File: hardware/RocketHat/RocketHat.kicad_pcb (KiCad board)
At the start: 4 copper layers, 28 x 25 mm, 32 parts, among them J1 Conn_02x16_Top_Bottom, J2 Conn_02x16_Top_Bottom, Q2 MMBT2222A, U1 BMP390, U2 BMI088, U3 ADXL375BCCZ, U5 74HC688, U6 74HC245, U7 74HC245, U8 MAX-M10S

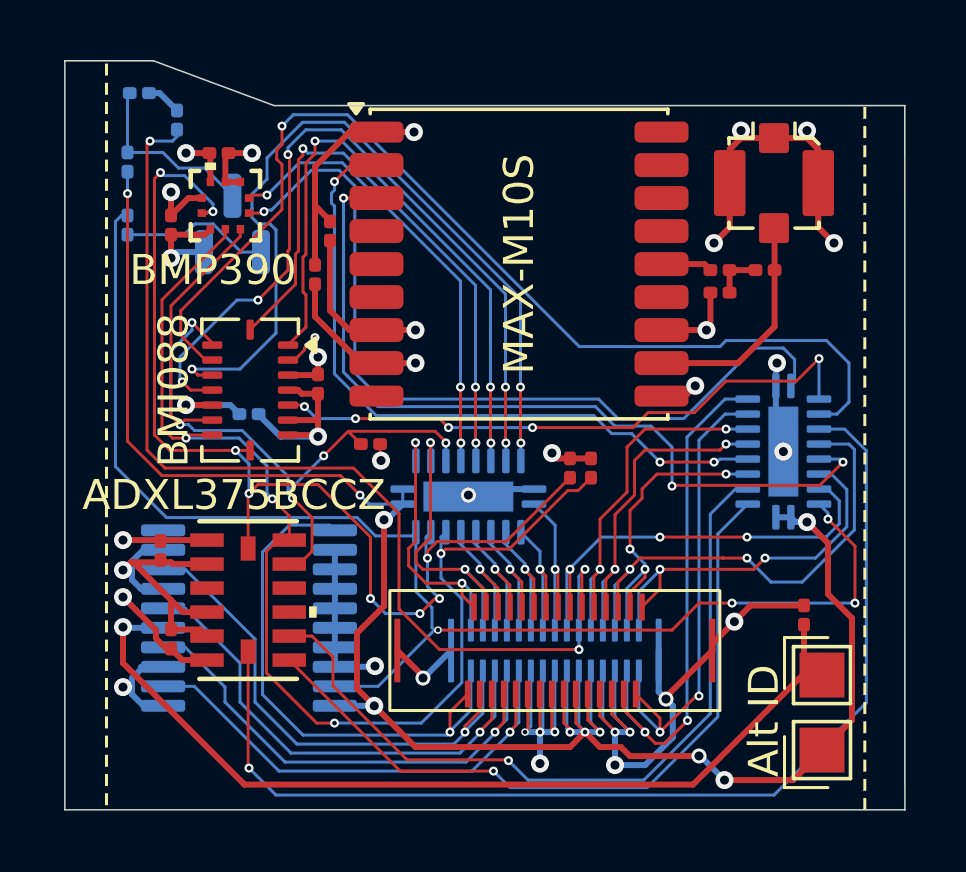
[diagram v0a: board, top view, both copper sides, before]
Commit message: sanity checked, ready for production
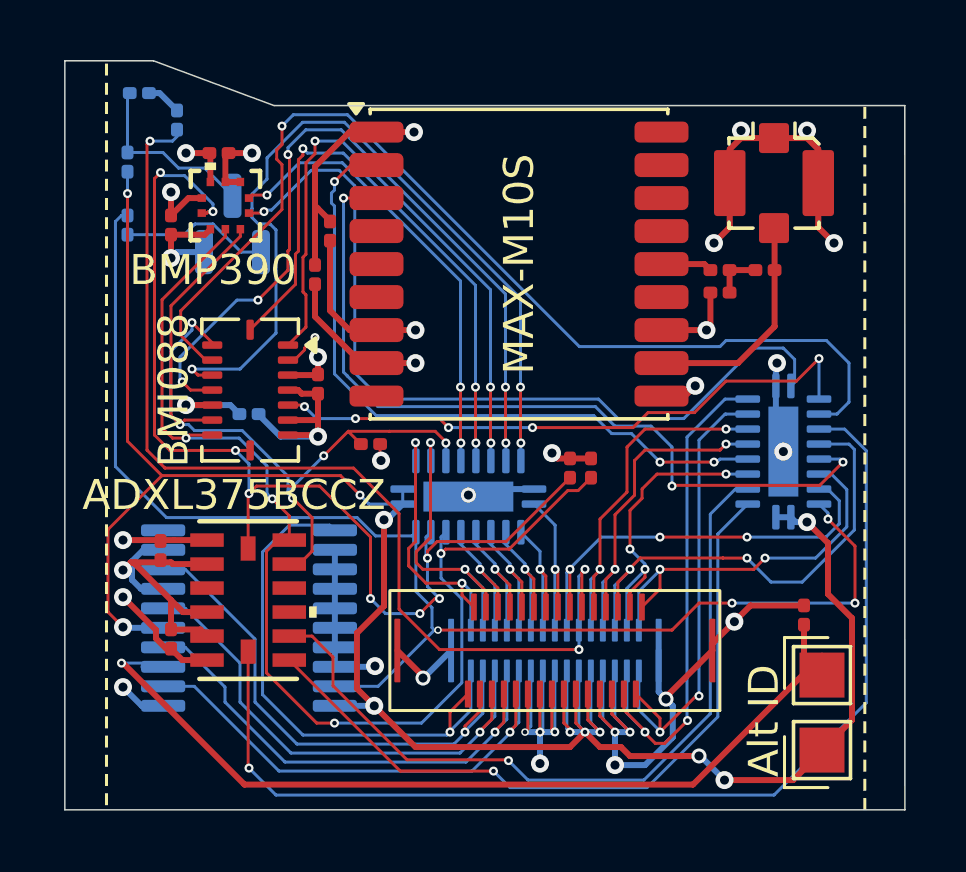
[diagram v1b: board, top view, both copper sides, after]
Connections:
- R8 pad 1: Net-(U5-R1) -> Net-(U5-R0)
- TP1 pad 1: Net-(U5-R1) -> Net-(U5-R0)
- U5 pad 3: CONN_26/GND -> Net-(U5-R0)
- U5 pad 5: Net-(U5-R1) -> CONN_23/5V
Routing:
- net Net-(U5-R1): track 31.2 -> 0.00 mm, vias 1 -> 0
- net Net-(U5-R0): track 0.00 -> 30.8 mm, vias 0 -> 1
- net CONN_23/5V: track 66.8 -> 74.2 mm, vias 10 -> 11
- net CONN_26/GND: track 87.4 -> 85.7 mm
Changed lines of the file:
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@@
 	(net 59 "CONN_2{slash}D2")
 	(net 60 "CONN_4{slash}D4")
-	(net 61 "Net-(U5-R1)")
+	(net 61 "Net-(U5-R0)")
 	(footprint "Capacitor_SMD:C_0201_0603Metric"
 		(layer "F.Cu")
@@
 			(size 1.5 1.5)
 			(layers "F.Cu" "F.Mask")
-			(net 61 "Net-(U5-R1)")
+			(net 61 "Net-(U5-R0)")
 			(pinfunction "1")
 			(pintype "passive")
@@
 			(layers "F.Cu" "F.Mask")
 			(roundrect_rratio 0.25)
-			(net 61 "Net-(U5-R1)")
+			(net 61 "Net-(U5-R0)")
 			(pintype "passive")
 		)
@@
 			(layers "B.Cu" "B.Mask" "B.Paste")
 			(roundrect_rratio 0.25)
-			(net 1 "CONN_26{slash}GND")
+			(net 61 "Net-(U5-R0)")
 			(pinfunction "R0")
 			(pintype "input")
@@
 			(layers "B.Cu" "B.Mask" "B.Paste")
 			(roundrect_rratio 0.25)
-			(net 61 "Net-(U5-R1)")
+			(net 5 "CONN_23{slash}5V")
 			(pinfunction "R1")
 			(pintype "input")
@@
 	)
 	(segment
-		(start 130.599 116.04387)
-		(end 130.599 115.8)
-		(width 0.2)
-		(layer "B.Cu")
-		(net 1)
-	)
-	(segment
 		(start 146.7 117.3)
 		(end 146.7 118.4)
@@
 	)
 	(segment
-		(start 130.599 115.8)
-		(end 130.3 115.8)
-		(width 0.2)
-		(layer "B.Cu")
-		(net 1)
-	)
-	(segment
 		(start 152.3125 107.95)
 		(end 152.0625 107.7)
@@
 	)
 	(segment
-		(start 130.599 115.50613)
-		(end 130.98013 115.125)
+		(start 147.702455 118.4)
+		(end 148.626 117.476455)
 		(width 0.2)
 		(layer "B.Cu")
@@
 	)
 	(segment
-		(start 147.702455 118.4)
-		(end 148.626 117.476455)
+		(start 131.6375 116.425)
+		(end 130.98013 116.425)
 		(width 0.2)
 		(layer "B.Cu")
@@
 	(segment
 		(start 131.6375 116.425)
-		(end 130.98013 116.425)
+		(end 130.925 116.425)
 		(width 0.2)
 		(layer "B.Cu")
@@
 	)
 	(segment
-		(start 130.98013 115.125)
-		(end 131.6375 115.125)
+		(start 130.925 116.425)
+		(end 130.3 115.8)
 		(width 0.2)
 		(layer "B.Cu")
@@
 	)
 	(segment
-		(start 131.6375 115.125)
-		(end 130.900001 115.125)
-		(width 0.2)
-		(layer "B.Cu")
-		(net 1)
-	)
-	(segment
 		(start 130.599 112.223999)
 		(end 130.599 111.9)
@@
 	)
 	(segment
-		(start 130.599 115.8)
-		(end 130.599 115.50613)
-		(width 0.2)
-		(layer "B.Cu")
-		(net 1)
-	)
-	(segment
 		(start 138.675 115.125)
 		(end 138.7 115.1)
@@
 	)
 	(segment
-		(start 130.98013 116.425)
-		(end 130.599 116.04387)
-		(width 0.2)
-		(layer "B.Cu")
-		(net 1)
-	)
-	(segment
 		(start 146.7 118.4)
 		(end 147.702455 118.4)
@@
 	)
 	(segment
+		(start 129.799 113.299)
+		(end 130.3 113.8)
+		(width 0.1)
+		(layer "F.Cu")
+		(net 5)
+	)
+	(segment
 		(start 130.45 107.604968)
 		(end 131.596032 108.751)
@@
 	)
 	(segment
+		(start 131.596032 108.751)
+		(end 129.799 110.548032)
+		(width 0.1)
+		(layer "F.Cu")
+		(net 5)
+	)
+	(segment
 		(start 147.2 118.1)
 		(end 146.899 117.799)
@@
 	)
 	(segment
+		(start 129.799 110.548032)
+		(end 129.799 113.299)
+		(width 0.1)
+		(layer "F.Cu")
+		(net 5)
+	)
+	(segment
 		(start 145.7953 116.8953)
 		(end 146.2 117.3)
@@
 	)
 	(via
+		(at 130.3 113.8)
+		(size 0.6)
+		(drill 0.3)
+		(layers "F.Cu" "B.Cu")
+		(net 5)
+	)
+	(via
 		(at 145.2 117.3)
 		(size 0.3)
@@
 	)
 	(segment
+		(start 130.325 113.825)
+		(end 130.3 113.8)
+		(width 0.2)
+		(layer "B.Cu")
+		(net 5)
+	)
+	(segment
 		(start 152.5625 110.1375)
 		(end 152.0625 110.1375)
@@
 	)
 	(segment
+		(start 131.6375 113.825)
+		(end 130.325 113.825)
+		(width 0.2)
+		(layer "B.Cu")
+		(net 5)
+	)
+	(segment
 		(start 152.5625 110.1375)
 		(end 152.725 110.3)
@@
 	)
 	(segment
+		(start 138.55 110.8)
+		(end 138.55 112.85)
+		(width 0.1)
+		(layer "F.Cu")
+		(net 25)
+	)
+	(segment
 		(start 140.45 111.268255)
 		(end 140.768255 110.95)
@@
 	)
 	(segment
+		(start 134.5 109.35)
+		(end 134.75 109.1)
+		(width 0.1)
+		(layer "F.Cu")
+		(net 25)
+	)
+	(segment
 		(start 131.55 98.65)
 		(end 131.35 98.85)
@@
 	)
 	(segment
-		(start 134.8 109.05)
-		(end 136.8 109.05)
-		(width 0.1)
-		(layer "F.Cu")
-		(net 25)
-	)
-	(segment
 		(start 140.768255 110.95)
 		(end 143.07 110.95)
@@
 	)
 	(segment
-		(start 134.5 109.35)
-		(end 134.8 109.05)
+		(start 134.75 109.1)
+		(end 136.85 109.1)
 		(width 0.1)
 		(layer "F.Cu")
@@
 	)
 	(segment
-		(start 136.8 109.05)
+		(start 136.85 109.1)
 		(end 138.55 110.8)
 		(width 0.1)
@@
 	)
 	(segment
-		(start 138.55 110.8)
-		(end 138.55 112.85)
-		(width 0.1)
-		(layer "F.Cu")
-		(net 25)
-	)
-	(segment
 		(start 131.35 107.4)
 		(end 131.8625 107.9125)
@@
 	)
 	(segment
-		(start 141.5943 115.650315)
-		(end 141.5943 112.863488)
+		(start 140.25 117)
+		(end 141.5943 115.6557)
 		(width 0.1)
 		(layer "B.Cu")
@@
 	)
 	(segment
-		(start 135.1 108.430755)
-		(end 134.169245 107.5)
+		(start 141.5943 112.863488)
+		(end 140.9 112.169188)
 		(width 0.1)
 		(layer "B.Cu")
@@
 	)
 	(segment
-		(start 135.1 109.35)
-		(end 135.1 108.430755)
+		(start 135.1 108.430755)
+		(end 134.169245 107.5)
 		(width 0.1)
 		(layer "B.Cu")
@@
 	)
 	(segment
-		(start 140.244615 117)
-		(end 141.5943 115.650315)
+		(start 135.1 109.35)
+		(end 135.1 108.430755)
 		(width 0.1)
 		(layer "B.Cu")
@@
 	)
 	(segment
-		(start 140.9 111.35)
-		(end 140.9 110.8)
+		(start 141.5943 115.6557)
+		(end 141.5943 112.863488)
 		(width 0.1)
 		(layer "B.Cu")
@@
 	)
 	(segment
-		(start 137.35 117)
-		(end 140.244615 117)
+		(start 140.9 112.169188)
+		(end 140.9 111.35)
 		(width 0.1)
 		(layer "B.Cu")
@@
 	)
 	(segment
-		(start 140.9 112.169188)
-		(end 140.9 111.35)
+		(start 140.9 111.35)
+		(end 140.9 110.8)
 		(width 0.1)
 		(layer "B.Cu")
@@
 	)
 	(segment
-		(start 141.5943 112.863488)
-		(end 140.9 112.169188)
+		(start 137.35 117)
+		(end 140.25 117)
 		(width 0.1)
 		(layer "B.Cu")
@@
 	)
 	(segment
-		(start 130.3 115)
-		(end 130.3 113.8)
+		(start 153 113.72)
+		(end 153 114.8)
 		(width 0.2)
 		(layer "F.Cu")
@@
 	)
 	(segment
-		(start 153 113.72)
-		(end 153 114.8)
-		(width 0.2)
+		(start 130.3 115)
+		(end 130.25 115)
+		(width 0.1)
 		(layer "F.Cu")
 		(net 61)
@@
 	)
 	(via
-		(at 130.3 113.8)
-		(size 0.6)
-		(drill 0.3)
+		(at 130.25 115)
+		(size 0.3)
+		(drill 0.15)
 		(layers "F.Cu" "B.Cu")
 		(net 61)
 	)
 	(segment
-		(start 130.325 113.825)
-		(end 130.3 113.8)
-		(width 0.2)
+		(start 130.25 115)
+		(end 131.5125 115)
+		(width 0.1)
 		(layer "B.Cu")
 		(net 61)
 	)
 	(segment
-		(start 131.6375 113.825)
-		(end 130.325 113.825)
+		(start 131.5125 115)
+		(end 131.6375 115.125)
+		(width 0.1)
+		(layer "B.Cu")
+		(net 61)
+	)
+	(segment
+		(start 130.98013 115.125)
+		(end 131.6375 115.125)
 		(width 0.2)
 		(layer "B.Cu")
